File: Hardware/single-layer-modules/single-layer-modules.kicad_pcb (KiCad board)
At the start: 2 copper layers, 150.5 x 90.5 mm, 20 parts, among them J1 Blue Pill - 1, J2 Blue Pill - 2, J3 SIM800L, J4 DS18B20, J5 DHT11, J6 FC-28, J7 MQ-02, J8 FC-37, Q1 FDS9435A, Q2 2N3904, SW1 SW_DIP_x05

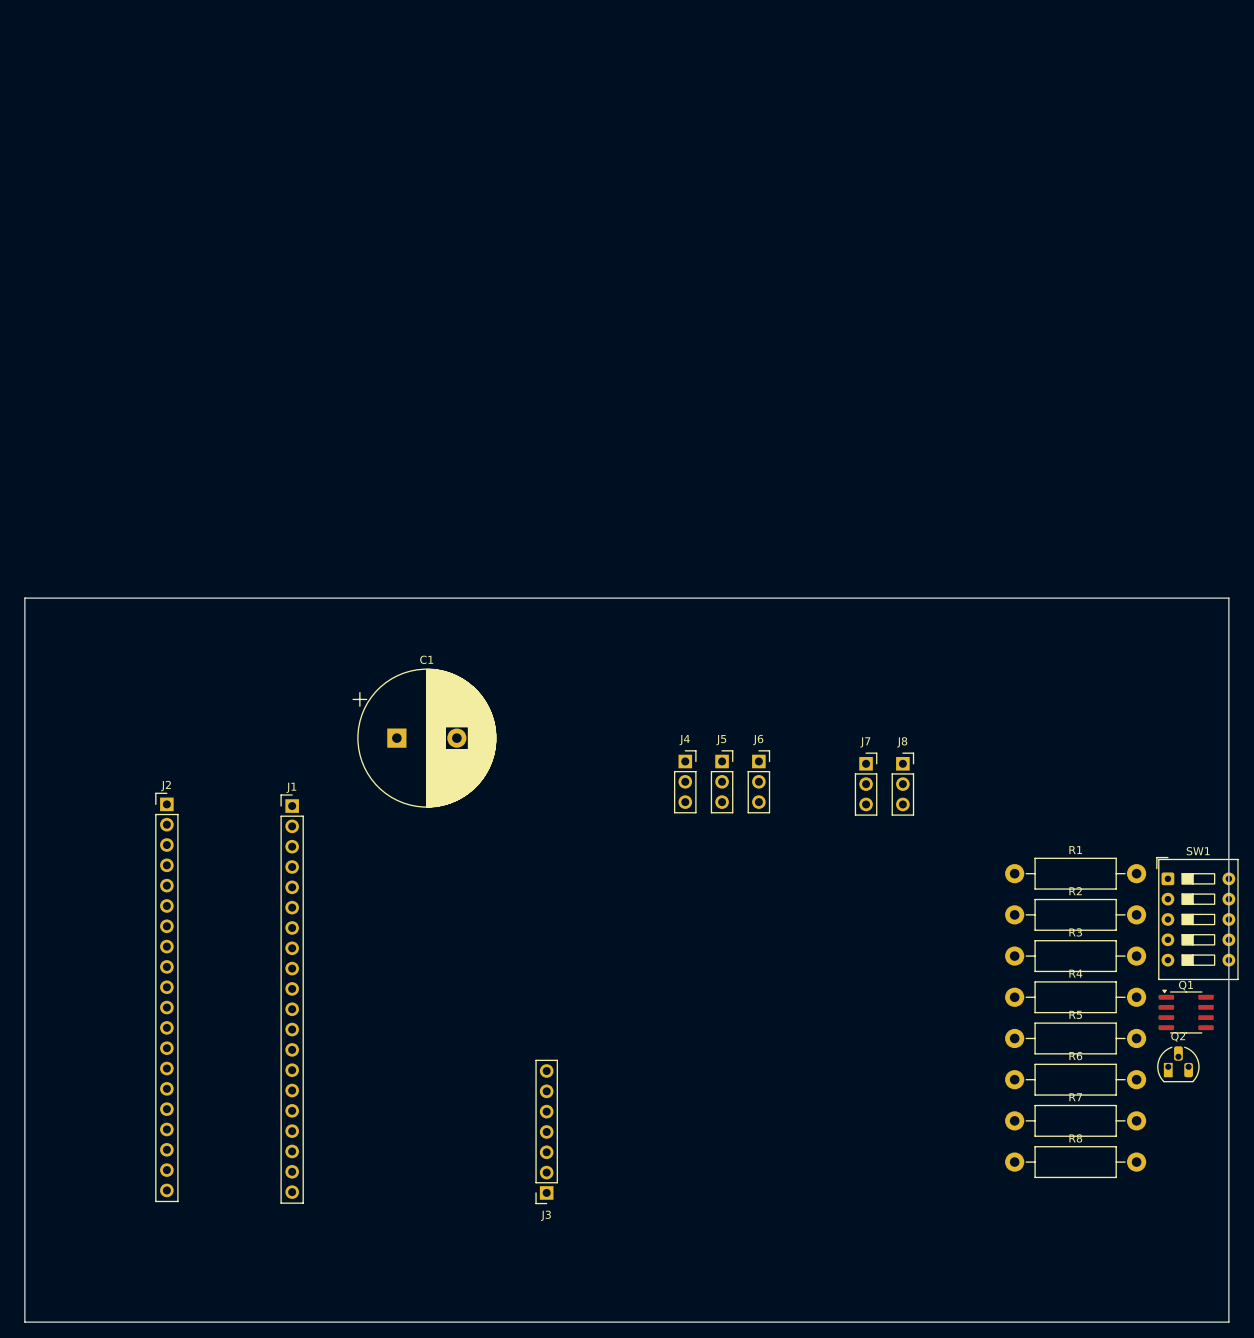
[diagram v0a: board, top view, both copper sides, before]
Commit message: Add New PCB
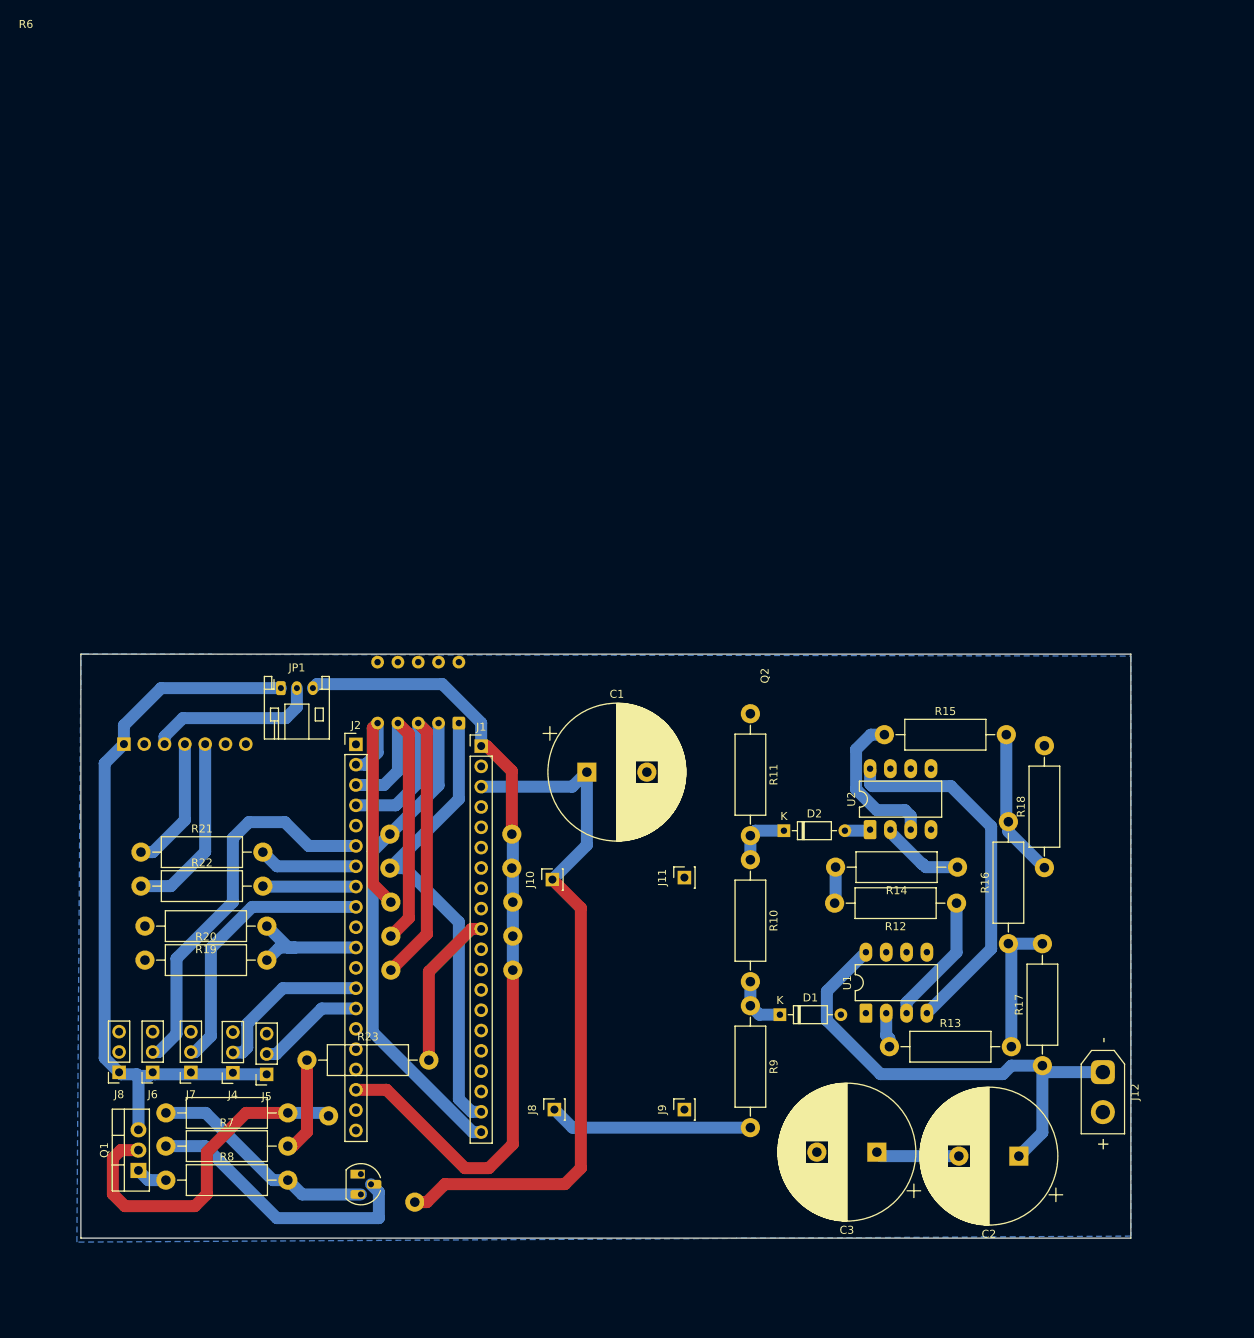
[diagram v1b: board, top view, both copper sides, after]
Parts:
- added C2: C_Polarized, Capacitor_THT:CP_Radial_D17.0mm_P7.50mm, F.Cu at (194.2, 98.5)
- added C3: C_Polarized, Capacitor_THT:CP_Radial_D17.0mm_P7.50mm, F.Cu at (176.5, 98.0)
- added D1: 1N4448, Diode_THT:D_DO-35_SOD27_P7.62mm_Horizontal, F.Cu at (164.4, 80.8)
- added D2: 1N4448, Diode_THT:D_DO-35_SOD27_P7.62mm_Horizontal, F.Cu at (164.9, 57.8)
- added J10: Conn_01x01_Pin, Connector_PinSocket_2.54mm:PinSocket_1x01_P2.54mm_Vertical, F.Cu at (135.9, 63.9)
- added J11: Conn_01x01_Pin, Connector_PinSocket_2.54mm:PinSocket_1x01_P2.54mm_Vertical, F.Cu at (152.4, 63.7)
- added J12: Conn_01x02_Socket, Connector_AMASS:AMASS_XT30UPB-M_1x02_P5.0mm_Vertical, F.Cu at (204.8, 88.0)
- added J8: Conn_01x01_Pin, Connector_PinSocket_2.54mm:PinSocket_1x01_P2.54mm_Vertical, F.Cu at (136.2, 92.7)
- added J9: Conn_01x01_Pin, Connector_PinSocket_2.54mm:PinSocket_1x01_P2.54mm_Vertical, F.Cu at (152.4, 92.7)
- added JP1: SolderJumper_3_Bridged12, Connector_JST:JST_PH_S3B-PH-K_1x03_P2.00mm_Horizontal, F.Cu at (102.0, 40.0)
- added R10: R, Resistor_THT:R_Axial_DIN0411_L9.9mm_D3.6mm_P15.24mm_Horizontal, F.Cu at (160.7, 61.4)
- added R11: R, Resistor_THT:R_Axial_DIN0411_L9.9mm_D3.6mm_P15.24mm_Horizontal, F.Cu at (160.7, 43.2)
- added R12: R, Resistor_THT:R_Axial_DIN0411_L9.9mm_D3.6mm_P15.24mm_Horizontal, F.Cu at (186.5, 66.9)
- added R13: R, Resistor_THT:R_Axial_DIN0411_L9.9mm_D3.6mm_P15.24mm_Horizontal, F.Cu at (178.1, 84.8)
- added R14: R, Resistor_THT:R_Axial_DIN0411_L9.9mm_D3.6mm_P15.24mm_Horizontal, F.Cu at (186.6, 62.4)
- added R15: R, Resistor_THT:R_Axial_DIN0411_L9.9mm_D3.6mm_P15.24mm_Horizontal, F.Cu at (177.4, 45.8)
- added R16: R, Resistor_THT:R_Axial_DIN0411_L9.9mm_D3.6mm_P15.24mm_Horizontal, F.Cu at (192.9, 71.9)
- added R17: R, Resistor_THT:R_Axial_DIN0411_L9.9mm_D3.6mm_P15.24mm_Horizontal, F.Cu at (197.2, 87.2)
- added R18: R, Resistor_THT:R_Axial_DIN0411_L9.9mm_D3.6mm_P15.24mm_Horizontal, F.Cu at (197.4, 62.4)
- added R19: R, Resistor_THT:R_Axial_DIN0411_L9.9mm_D3.6mm_P15.24mm_Horizontal, F.Cu at (100.2, 69.8)
- added R20: R, Resistor_THT:R_Axial_DIN0411_L9.9mm_D3.6mm_P15.24mm_Horizontal, F.Cu at (85.0, 74.0)
- added R21: R, Resistor_THT:R_Axial_DIN0411_L9.9mm_D3.6mm_P15.24mm_Horizontal, F.Cu at (84.5, 60.5)
- added R22: R, Resistor_THT:R_Axial_DIN0411_L9.9mm_D3.6mm_P15.24mm_Horizontal, F.Cu at (84.5, 64.8)
- added R23: R, Resistor_THT:R_Axial_DIN0411_L9.9mm_D3.6mm_P15.24mm_Horizontal, F.Cu at (105.3, 86.5)
- added R24: R, Resistor_THT:R_Axial_DIN0411_L9.9mm_D3.6mm_P15.24mm_Horizontal, B.Cu at (118.7, 104.2)
- added R9: R, Resistor_THT:R_Axial_DIN0411_L9.9mm_D3.6mm_P15.24mm_Horizontal, F.Cu at (160.7, 79.7)
- added U1: LM358, Package_DIP:DIP-8_W7.62mm_LongPads, F.Cu at (175.1, 80.6)
- added U2: LM358, Package_DIP:DIP-8_W7.62mm_LongPads, F.Cu at (175.7, 57.7)
- J3, R1, R2, R3, R4, R5, SW1: moved to B.Cu
- Q1: value FDS9435A -> IRF4905; footprint Package_SO:SOIC-8_3.9x4.9mm_P1.27mm -> Package_TO_SOT_THT:TO-220-3_Vertical
- moved Q1 132.5 mm to (84.2, 100.3), turned to 90 degrees
- moved R6 106.2 mm to (87.6, 93.1)
- moved R7 106.1 mm to (87.6, 97.2)
- moved R8 106.1 mm to (87.6, 101.5)
- moved J8 105.3 mm to (81.8, 88.0), turned to 180 degrees
- moved Q2 101.8 mm to (112.0, 100.8), turned to -90 degrees
- moved J7 92.8 mm to (90.8, 88.0), turned to 180 degrees
- moved SW1 90.7 mm to (124.2, 44.4), turned to 90 degrees
- moved J6 85.2 mm to (86.0, 88.0), turned to 180 degrees
- moved R5 79.8 mm to (115.8, 66.8)
- moved R2 78.7 mm to (115.6, 58.2)
- moved R4 78.3 mm to (115.8, 71.0)
- moved R1 78.1 mm to (115.6, 62.5)
- moved R3 78.0 mm to (115.8, 75.2)
- moved J3 77.1 mm to (82.4, 47.0), turned to -90 degrees
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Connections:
- J1 pad 10: unconnected-(J1-Pin_10-Pad10) -> PB_3
- J1 pad 11: unconnected-(J1-Pin_11-Pad11) -> PA_15
- J1 pad 12: unconnected-(J1-Pin_12-Pad12) -> PA_12
- J1 pad 13: unconnected-(J1-Pin_13-Pad13) -> PA_11
- J1 pad 14: unconnected-(J1-Pin_14-Pad14) -> PA_10
- J1 pad 15: unconnected-(J1-Pin_15-Pad15) -> PA_9
- J1 pad 16: unconnected-(J1-Pin_16-Pad16) -> PA_8
- J1 pad 17: unconnected-(J1-Pin_17-Pad17) -> PB_15
- J1 pad 18: unconnected-(J1-Pin_18-Pad18) -> PB_14
- J1 pad 19: unconnected-(J1-Pin_19-Pad19) -> PB_13
- J1 pad 20: PB_1 -> PB_12
- J1 pad 4: unconnected-(J1-Pin_4-Pad4) -> PB_9
- J1 pad 5: unconnected-(J1-Pin_5-Pad5) -> PB_8
- J1 pad 6: unconnected-(J1-Pin_6-Pad6) -> PB_7
- J1 pad 7: unconnected-(J1-Pin_7-Pad7) -> PB_6
- J1 pad 8: unconnected-(J1-Pin_8-Pad8) -> PB_5
- J1 pad 9: unconnected-(J1-Pin_9-Pad9) -> PB_4
- J3 pad 3: VCC_5V -> SIM800L
- J3 pad 4: unconnected-(J3-Pin_4-Pad4) -> Net-(J3-Pin_4)
- J3 pad 5: unconnected-(J3-Pin_5-Pad5) -> Net-(J3-Pin_5)
- J4 pad 2: unconnected-(J4-Pin_2-Pad2) -> PB_0
- J5 pad 2: unconnected-(J5-Pin_2-Pad2) -> PB_1
- J6 pad 2: unconnected-(J6-Pin_2-Pad2) -> PA_1
- J7 pad 2: unconnected-(J7-Pin_2-Pad2) -> PA_4
- Q1 pad 1: VCC_5V -> Net-(Q1-G)
- Q1 pad 2: VCC_5V -> +5V
- R1 pad 1: Net-(R1-Pad1) -> PB_13
- R2 pad 1: Net-(R2-Pad1) -> PB_12
- R3 pad 1: Net-(R3-Pad1) -> PC_15
- R4 pad 1: Net-(R4-Pad1) -> PC_14
- R5 pad 1: Net-(R5-Pad1) -> PC_13
- R7 pad 2: unconnected-(R7-Pad2) -> Net-(R23-Pad1)
- SW1 pad 1: Net-(R1-Pad1) -> PB_13
- SW1 pad 2: Net-(R2-Pad1) -> PB_12
- SW1 pad 3: Net-(R3-Pad1) -> PC_15
- SW1 pad 4: Net-(R4-Pad1) -> PC_14
- SW1 pad 5: Net-(R5-Pad1) -> PC_13
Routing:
- net +5V: track 0.00 -> 133.0 mm
- net +3.3V: track 0.00 -> 102.9 mm
- net VCC_5V: track 0.00 -> 92.3 mm
- net SOLAR_REG_IN: track 0.00 -> 61.1 mm
- net PB_12: track 0.00 -> 60.8 mm
- net PB_13: track 0.00 -> 58.7 mm
- net PC_15: track 0.00 -> 49.6 mm
- net PA_1: track 0.00 -> 48.8 mm
- net Net-(U1C-V-): track 0.00 -> 45.9 mm
- net PC_14: track 0.00 -> 40.1 mm
- net Net-(Q2-B): track 0.00 -> 35.0 mm
- net PA_4: track 0.00 -> 34.6 mm
- net PC_13: track 0.00 -> 30.6 mm
- net Net-(Q2-C): track 0.00 -> 28.6 mm
- net VCC_IN: track 0.00 -> 25.4 mm
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- added copper zone on B.Cu, net GND
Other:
- board size 150.5 x 90.5 mm -> 131.2 x 73 mm
